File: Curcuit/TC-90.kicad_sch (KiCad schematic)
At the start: 8 parts, among them Q1 2N3904, Q2 50N06

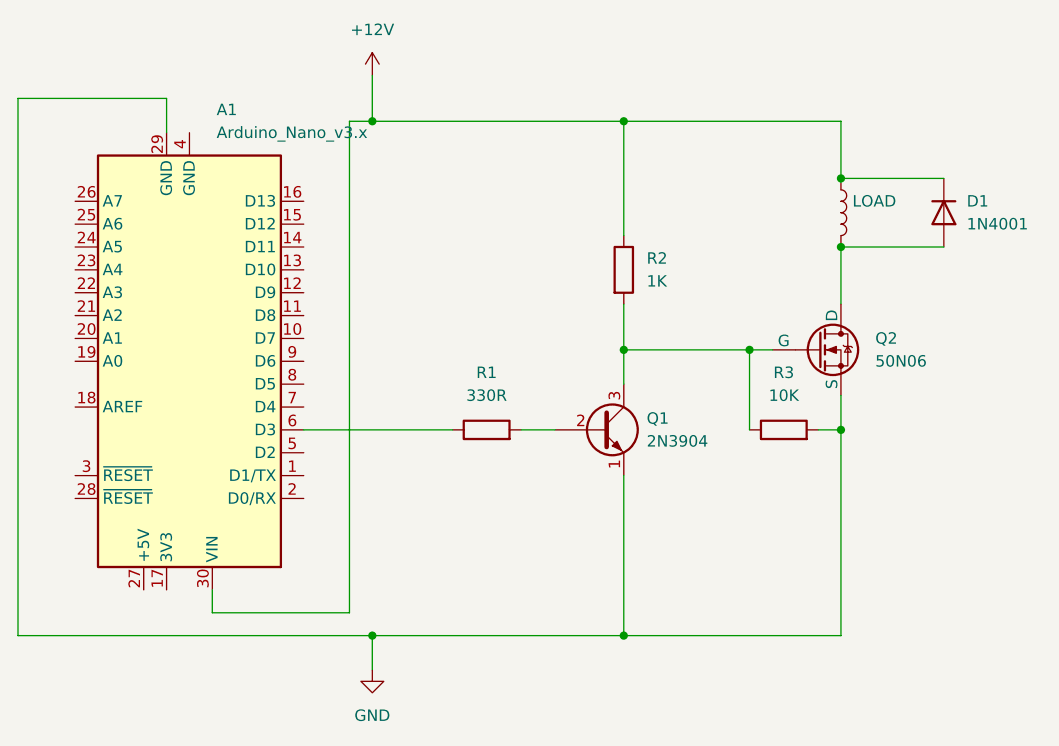
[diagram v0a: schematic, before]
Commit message: Added pics
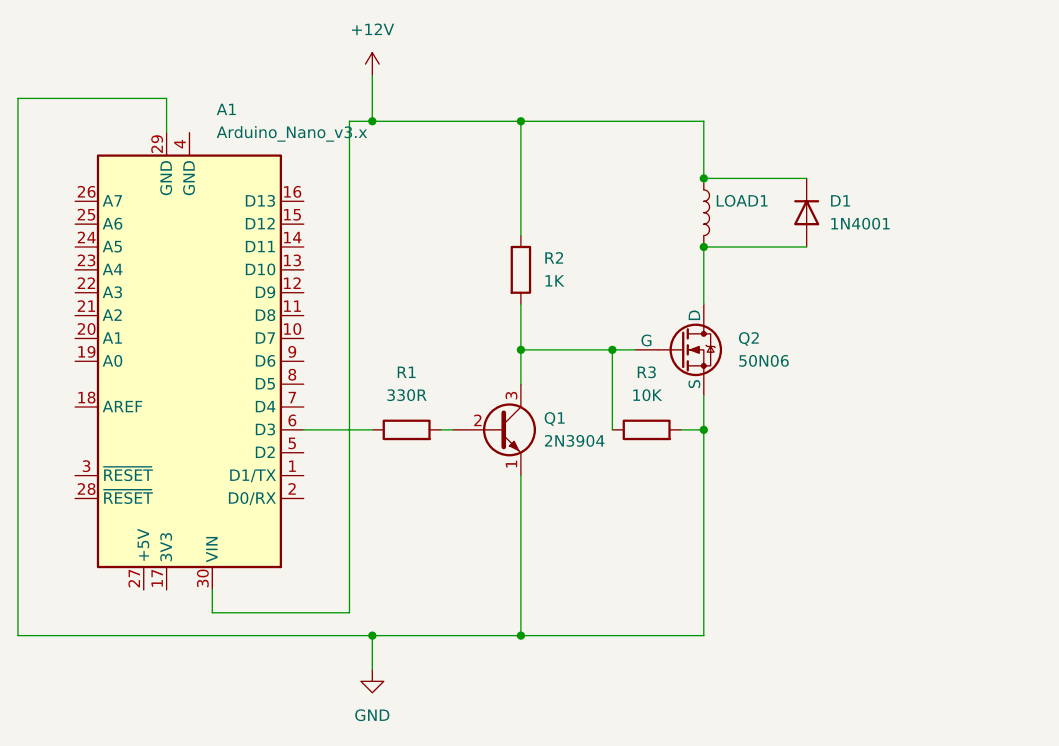
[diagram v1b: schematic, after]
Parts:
- renumbered LOAD to LOAD1
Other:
- moved on the sheet: D1, LOAD1, Q1, Q2, R1, R2, R3
